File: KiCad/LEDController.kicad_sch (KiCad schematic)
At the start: 41 parts, among them SW1 BOOT, SW2 EN, U1 TPS54202DDC, U2 ESP32-S3-WROOM-2, U3 TPS54202DDC

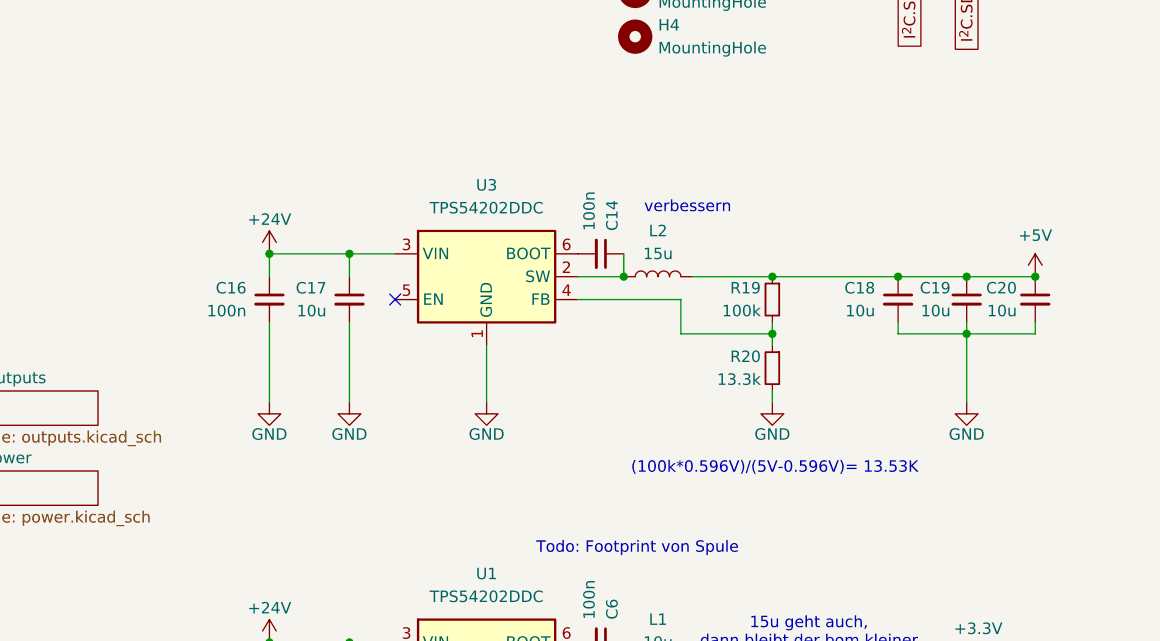
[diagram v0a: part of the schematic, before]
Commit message: work on new design
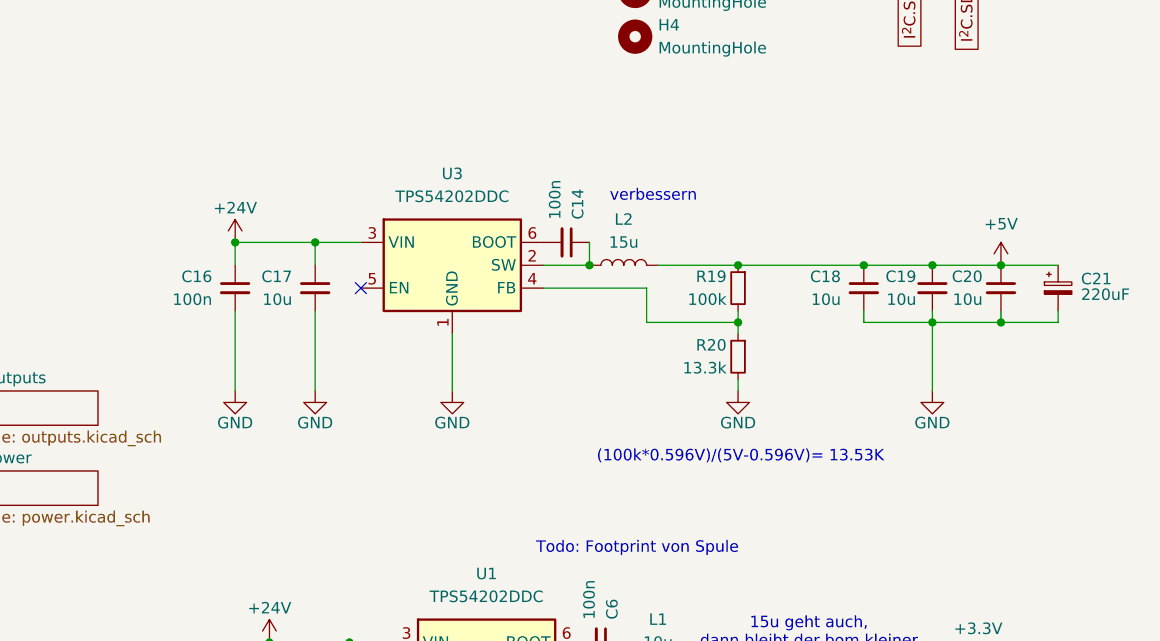
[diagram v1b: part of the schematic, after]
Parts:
- added C21: 220uF, Capacitor_THT:CP_Radial_D8.0mm_P3.50mm, symbol Device:C_Polarized_Small
- L2: footprint Inductor_SMD:L_APV_ANR4026 -> Inductor_SMD:L_APV_APH0420
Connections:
- net +5V: now also C21.1
- net GND: now also C21.2
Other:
- moved on the sheet: C14, C16, C17, C18, C19, C20, L2, R19, R20, U3
